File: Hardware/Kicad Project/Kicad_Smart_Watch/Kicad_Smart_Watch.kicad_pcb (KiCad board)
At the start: 2 copper layers, 31 x 26.4 mm, 55 parts, among them J1 Conn2, J3 FPC, Q1 MMBT3904, SW1 SW_Push, SW2 SW_Push, SW3 SW_Push, SW4 SW_Push, U1 RV-3028-C7, U3 USB-AB, U4 TPS62840DLCR, U5 ATMEGA32U4QFN, Y1 16MHz

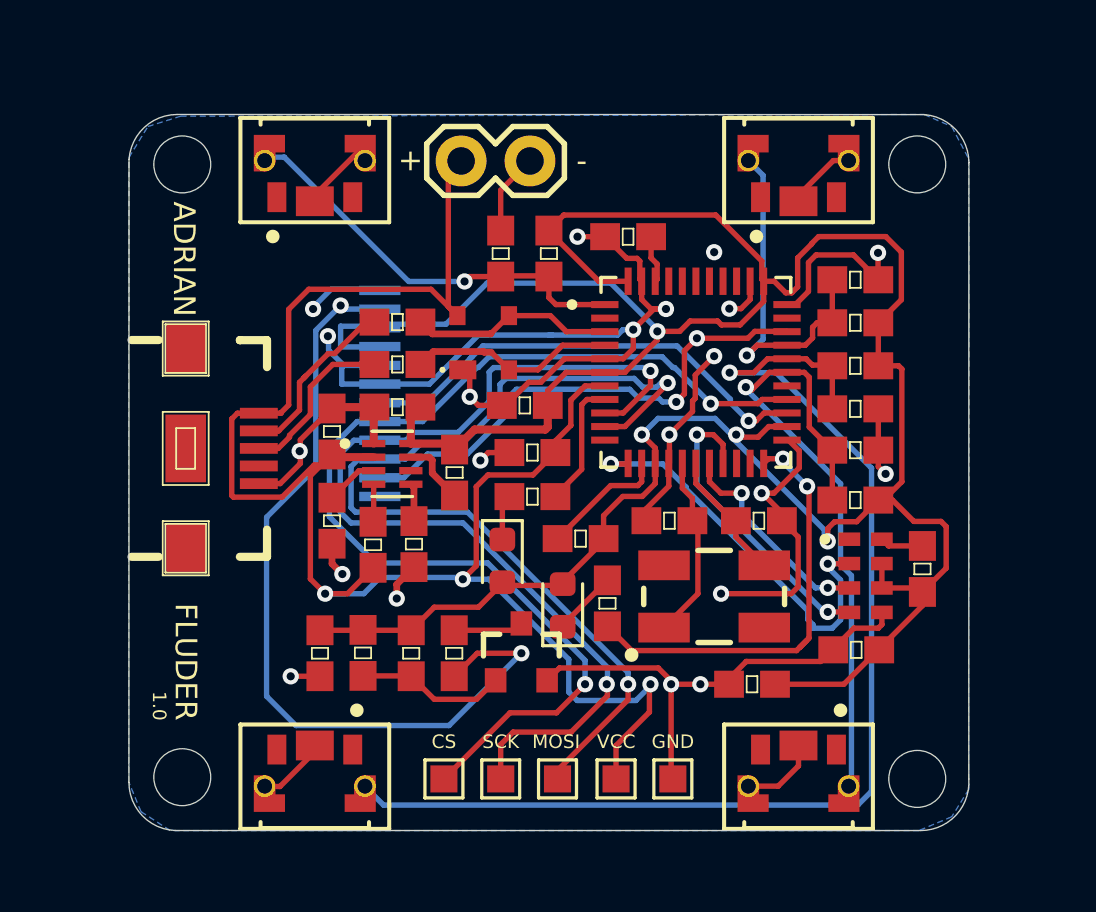
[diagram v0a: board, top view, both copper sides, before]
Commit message: updated mcu board pcb
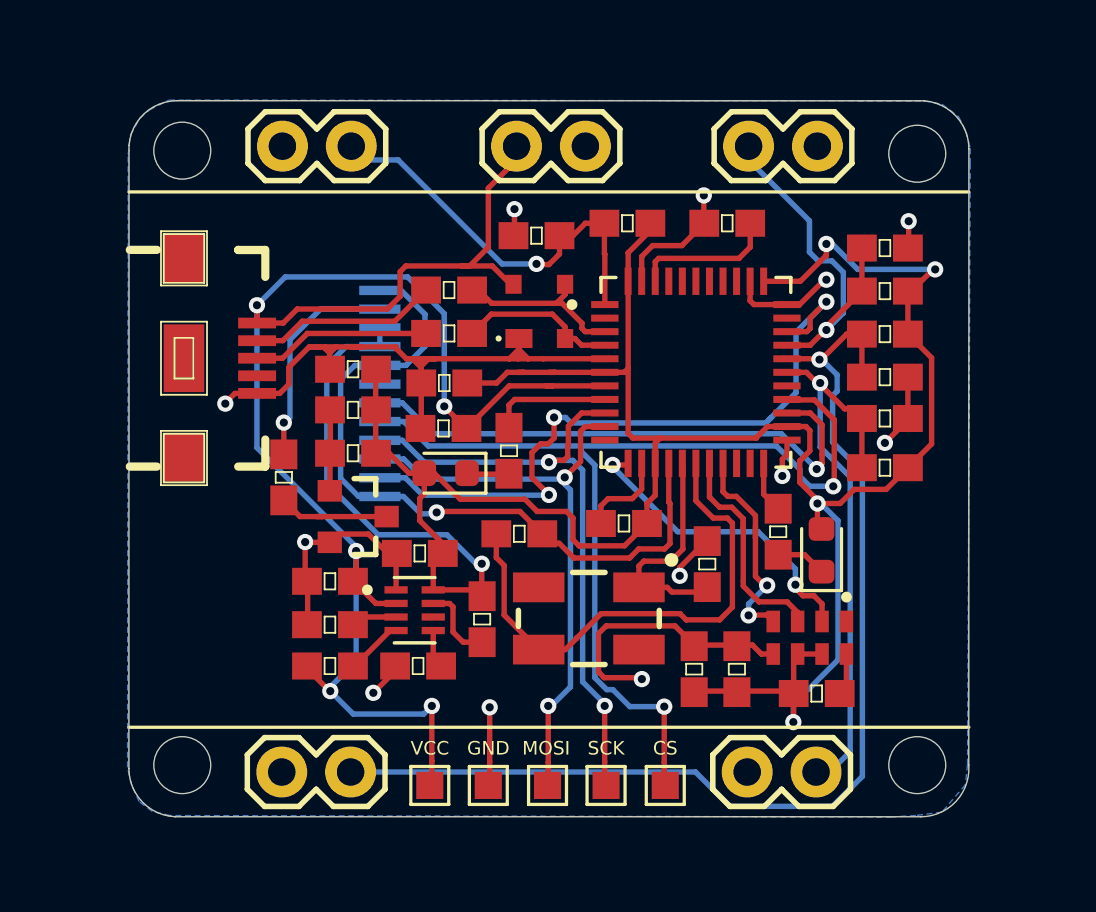
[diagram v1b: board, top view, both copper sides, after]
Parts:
- removed the REF** at (88.3, 73.0)
- removed the REF** at (88.3, 95.6)
- removed the REF** at (115.4, 95.6)
- added REF**: MountingHole_2.1mm, MountingHole:MountingHole_2.1mm, F.Cu at (88.3, 72.5)
- added REF**: MountingHole_2.1mm, MountingHole:MountingHole_2.1mm, F.Cu at (88.3, 95.1)
- added REF**: MountingHole_2.1mm, MountingHole:MountingHole_2.1mm, F.Cu at (115.4, 95.1)
- SW1, SW2, SW3, SW4: footprint Downloads:Panasonic-EVP-AKE31A-MFG -> Downloads:1X02
- moved C7 10.5 mm to (94.6, 80.5), turned to 180 degrees
- moved D2 9.76 mm to (111.9, 87.2)
- moved R8 9.04 mm to (92.1, 84.5), turned to 270 degrees
- moved R1 8.97 mm to (94.6, 82.0), turned to 0 degrees
- moved C5 8.85 mm to (100.8, 86.6)
- moved CS 8.17 mm to (106.1, 95.9)
- moved Q1 7.89 mm to (94.8, 86.0), turned to 270 degrees
- moved R3 7.68 mm to (94.6, 83.6), turned to 0 degrees
- moved VCC 6.87 mm to (97.5, 95.9)
- moved R6 6.83 mm to (110.3, 86.5), turned to 270 degrees
- moved GND 6.81 mm to (99.6, 95.9)
- moved R9 6.03 mm to (111.7, 92.5), turned to 0 degrees
- moved C1 6.02 mm to (107.2, 91.6), turned to 90 degrees
- moved C17 5.53 mm to (93.8, 88.3), turned to 180 degrees
- moved L1 5.50 mm to (99.4, 89.7)
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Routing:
- net /LEDK: track 30.9 -> 7.85 mm, vias 2 -> 1
- net Net-(C5-Pad1): track 4.86 -> 20.3 mm
- net Net-(R6-Pad1): track 16.2 -> 1.89 mm, vias 2 -> 0
- net /SCK: track 37.5 -> 23.2 mm
- net GND: track 105.6 -> 91.4 mm, vias 21 -> 13
- net /MOSI: track 35.8 -> 21.9 mm
- net 3.3V: track 112.5 -> 104.2 mm, vias 4 -> 5
- net /D5: track 18.9 -> 25.7 mm, vias 2 -> 3
- net /D12: track 40.7 -> 36.9 mm
- net /AREF: track 1.77 -> 5.23 mm
- net /D11: track 15.2 -> 12.0 mm
- net /D4: track 17.5 -> 20.3 mm
- net VCC: track 65.5 -> 62.7 mm, vias 3 -> 5
- net /D2: track 11.1 -> 8.31 mm
- net Net-(Q1-Pad1): track 5.54 -> 3.00 mm
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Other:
- board text removed: "+"
- board text removed: "-"
- board text removed: "1.0"
- board text removed: "ADRIAN"
- board text removed: "FLUDER"

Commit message: update
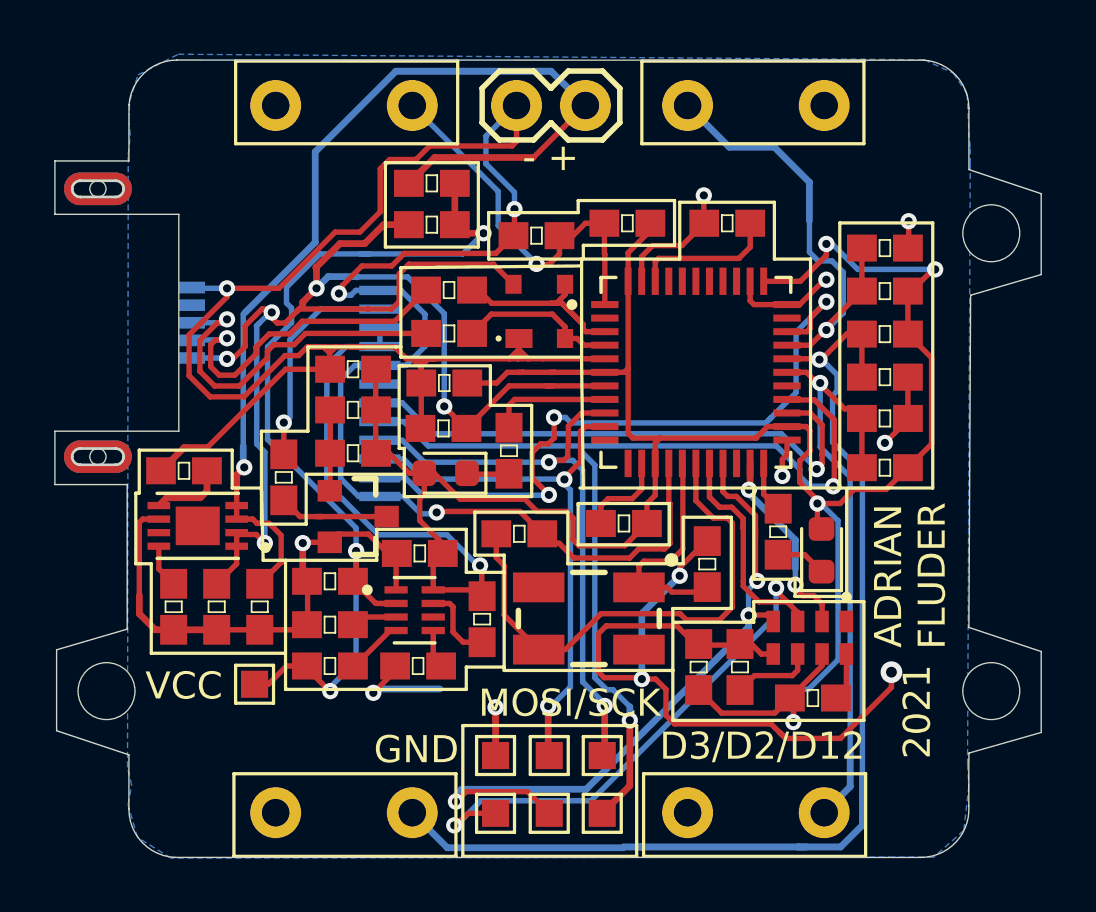
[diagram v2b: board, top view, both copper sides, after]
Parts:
- removed C1: 100nF, Downloads:0603
- removed the REF** at (88.3, 72.5)
- removed the REF** at (88.3, 95.1)
- removed the REF** at (115.4, 95.1)
- removed the REF** at (115.4, 72.6)
- added C3: 4.7uF, Downloads:0603, F.Cu at (89.6, 89.3)
- added C4: 4.7uF, Downloads:0603, F.Cu at (91.2, 89.3)
- added D1: D_Schottky, Downloads:0603, F.Cu at (97.5, 75.2)
- added D5: D_Schottky, Downloads:0603, F.Cu at (97.5, 73.7)
- added D6: LED, Downloads:0603, F.Cu at (88.4, 84.3)
- added Q2: MCP73831_2, Downloads:SON50P200X300X100-9N, F.Cu at (88.9, 86.3)
- added R17: 2k, Downloads:0603, F.Cu at (88.0, 89.3)
- added R18: 10k, Downloads:0603, F.Cu at (108.9, 91.5)
- added REF**: MountingHole_2.1mm, MountingHole:MountingHole_2.1mm, F.Cu at (118.2, 75.5)
- added REF**: MountingHole_2.1mm, MountingHole:MountingHole_2.1mm, F.Cu at (118.2, 92.4)
- added REF**: MountingHole_2.1mm, MountingHole:MountingHole_2.1mm, F.Cu at (85.5, 92.4)
- added TP4: TestPoint, TestPoint:TestPoint_Pad_1.0x1.0mm, F.Cu at (99.9, 96.9)
- added TP5: TestPoint, TestPoint:TestPoint_Pad_1.0x1.0mm, F.Cu at (101.9, 96.9)
- R9: value R -> 10k
- U3: footprint Downloads:USB-AB-MICRO-SMD -> Downloads:GCT_USB3155-XX-X_REVA; moved to B.Cu
- moved VCC 7.47 mm to (91.0, 92.1)
- moved U3 3.43 mm to (85.2, 78.8), turned to 90 degrees
- moved TP1 2.54 mm to (103.8, 96.9)
- moved SW3 1.82 mm to (95.6, 96.9)
- moved SW2 1.80 mm to (95.6, 70.8)
- moved SW4 1.80 mm to (108.2, 70.8)
- moved SW1 1.78 mm to (110.8, 96.9)
- moved J1 1.50 mm to (100.7, 70.8)
- moved C2 1.41 mm to (107.4, 91.5)
- moved GND 1.14 mm to (99.9, 94.8)
- moved TP3 1.11 mm to (103.8, 94.8)
- moved TP2 1.11 mm to (101.9, 94.8)
- moved R9 0.22 mm to (111.6, 92.6)
- renumbered CS to TP1, MOSI to TP2, SCK to TP3
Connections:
- net /A3 renamed Net-(U5-Pad39)
- net /A4 renamed Net-(U5-Pad40)
- net /A5 renamed Net-(U5-Pad41)
- C12 pad 1: VCC -> VBUS
- D4 pad 4: VCC -> VBUS
- J1 pad 1: VCC -> GND
- J1 pad 2: GND -> /BAT+
- U1 pad 2: /D11 -> /INT
- U1 pad 6: 3.3V -> Net-(R18-Pad1)
- U3 pad VBUS: VCC -> VBUS
- U5 pad 21: /TXO -> /INT
- U5 pad 7: VCC -> VBUS
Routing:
- net GND: track 91.4 -> 163.2 mm, vias 13 -> 15
- net VBUS: track 0.00 -> 50.0 mm, vias 0 -> 5
- net /BAT+: track 0.00 -> 45.7 mm, vias 0 -> 1
- net VCC: track 62.7 -> 34.7 mm, vias 5 -> 3
- net /D3: track 8.31 -> 27.0 mm, vias 0 -> 2
- net /D2: track 8.31 -> 26.0 mm, vias 2 -> 3
- net /D11: track 12.0 -> 0.41 mm, vias 2 -> 0
- net /INT: track 0.00 -> 6.94 mm, vias 0 -> 2
- net Net-(R7-Pad2): track 6.59 -> 13.0 mm, vias 0 -> 1
- net Net-(R5-Pad2): track 7.06 -> 12.2 mm, vias 0 -> 1
- net /BTN2: track 13.9 -> 17.8 mm
- net Net-(R18-Pad1): track 0.00 -> 3.24 mm
- net Net-(D6-Pad2): track 0.00 -> 3.12 mm
- net Net-(Q2-Pad8): track 0.00 -> 1.61 mm
- net /D-: track 6.48 -> 7.91 mm
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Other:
- board size 31 x 26.4 mm -> 36.4 x 29.4 mm
- board text added: "- +"
- board text added: "2021"
- board text added: "ADRIAN FLUDER"
- board text added: "D3/D2/D12"
- board text added: "GND"
- board text added: "MOSI/SCK"
- board text added: "VCC"
